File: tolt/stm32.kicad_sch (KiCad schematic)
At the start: 16 parts, among them U1 STM32F405RGTx, Y1 8m

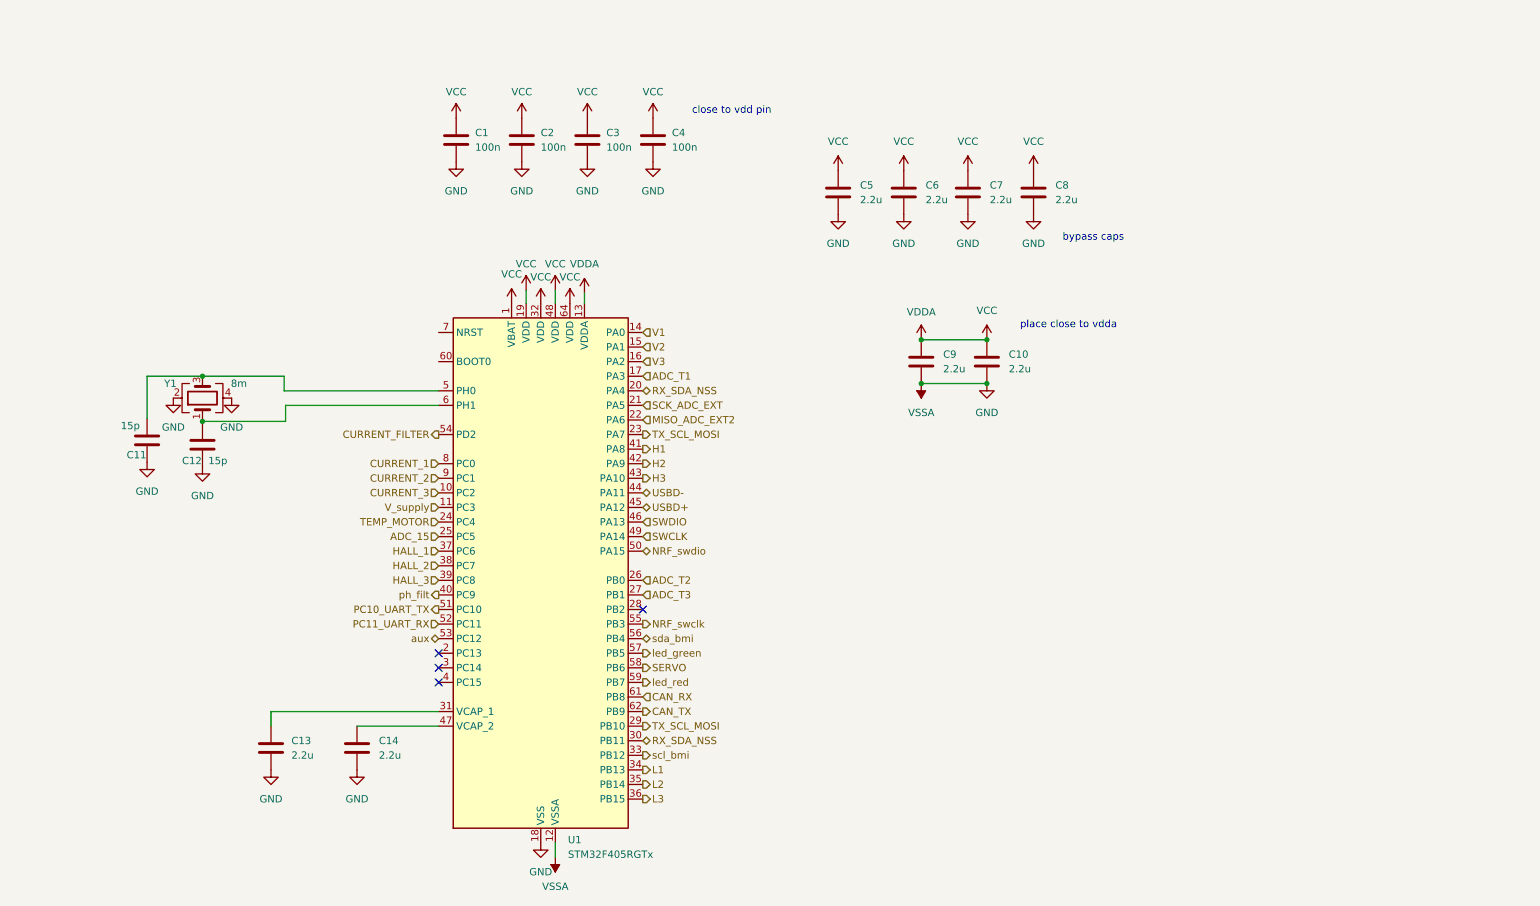
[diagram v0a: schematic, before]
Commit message: new file:   tolt/powerstage.kicad_sch 	modified:   tolt/stm32.kicad_sch 	modified:   tolt/tolt.kicad_pro 	modified:   tolt/tolt.kicad_sch
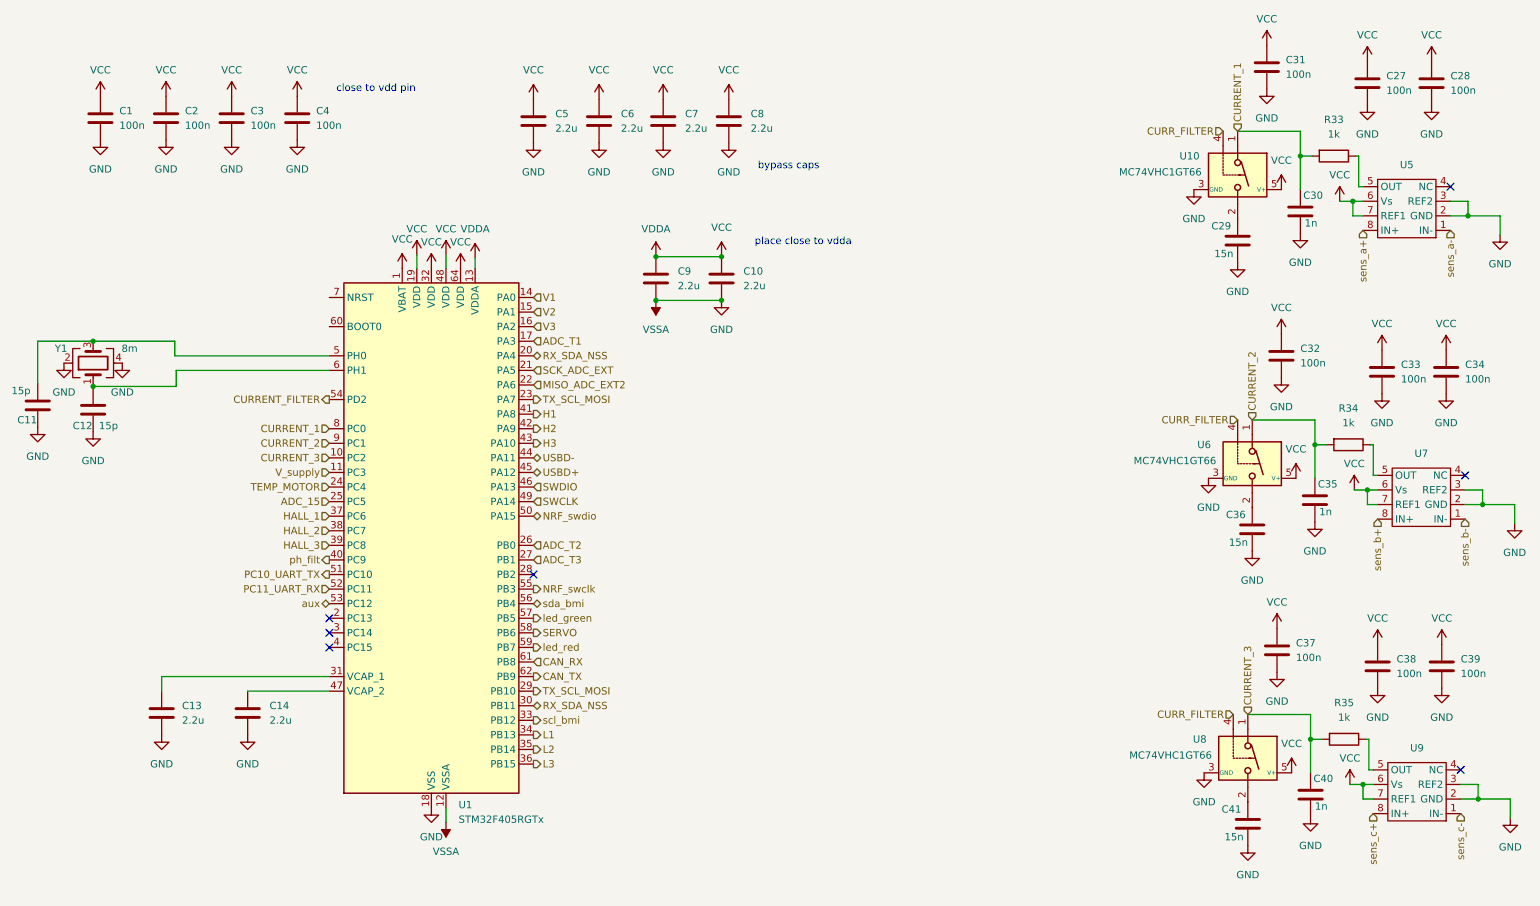
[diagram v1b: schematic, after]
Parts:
- added C27, C28, C31, C32, C33, C34, C37, C38, C39: 100n, Capacitor_SMD:C_0402_1005Metric, symbol Device:C
- added C29, C36, C41: 15n, Capacitor_SMD:C_0603_1608Metric, symbol Device:C
- added C30, C35, C40: 1n, Capacitor_SMD:C_0603_1608Metric, symbol Device:C
- added R33, R34, R35: 1k, Resistor_SMD:R_0603_1608Metric, symbol Device:R
- added U10, U6, U8: MC74VHC1GT66, Package_TO_SOT_SMD:SOT-353_SC-70-5, symbol Analog_Switch:TS5A3166DCKR
- added U5, U7, U9: ~, Package_TO_SOT_SMD:SOT-23-8, symbol Amplifier_Current:INA241
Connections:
- net CURRENT_1: now also C30.1, R33.2, U10.1
- net CURRENT_2: now also C35.1, R34.2, U6.1
- net CURRENT_3: now also C40.1, R35.2, U8.1
- net GND: now also C27.1, C28.1, C29.2, C30.2, C31.1, C32.1, C33.1, C34.1, C35.2, C36.2, C37.1, C38.1, C39.1, C40.2, C41.2, U10.3 (GND), U5.2 (GND), U5.3 (REF2), U6.3 (GND), U7.2 (GND), U7.3 (REF2), U8.3 (GND), U9.2 (GND), U9.3 (REF2)
- net VCC: now also C27.2, C28.2, C31.2, C32.2, C33.2, C34.2, C37.2, C38.2, C39.2, U10.5 (V+), U5.6 (Vs), U5.7 (REF1), U6.5 (V+), U7.6 (Vs), U7.7 (REF1), U8.5 (V+), U9.6 (Vs), U9.7 (REF1)
- new net: R33.1, U5.5 (OUT)
- new net: C36.1, U6.2
- new net: R34.1, U7.5 (OUT)
- new net: C29.1, U10.2
- new net: R35.1, U9.5 (OUT)
- new net: C41.1, U8.2
- new net CURR_FILTER: U10.4, U6.4, U8.4
- new net sens_a+: U5.8 (IN+)
- new net sens_a-: U5.1 (IN-)
- new net sens_b+: U7.8 (IN+)
- new net sens_b-: U7.1 (IN-)
- new net sens_c+: U9.8 (IN+)
- new net sens_c-: U9.1 (IN-)
- no-connect marks 4 -> 7
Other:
- moved on the sheet: C1, C10, C11, C12, C13, C14, C2, C3, C4, C5, C6, C7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
